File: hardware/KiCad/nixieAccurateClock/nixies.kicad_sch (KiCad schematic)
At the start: 7 parts, among them J17 Conn_02x05_Odd_Even

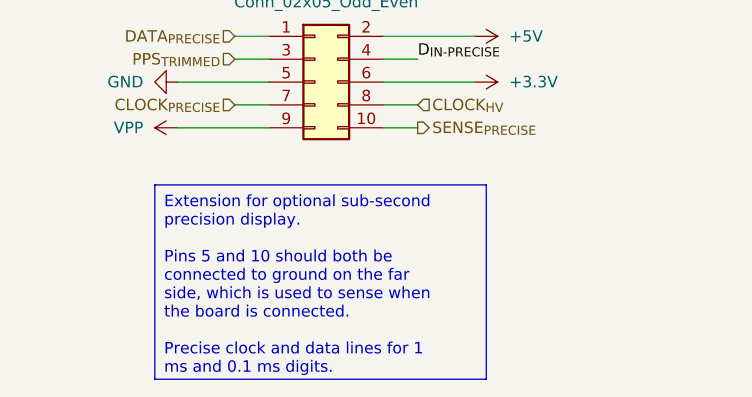
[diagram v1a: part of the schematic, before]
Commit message: Modify HV supply to attempt to solve weak IC
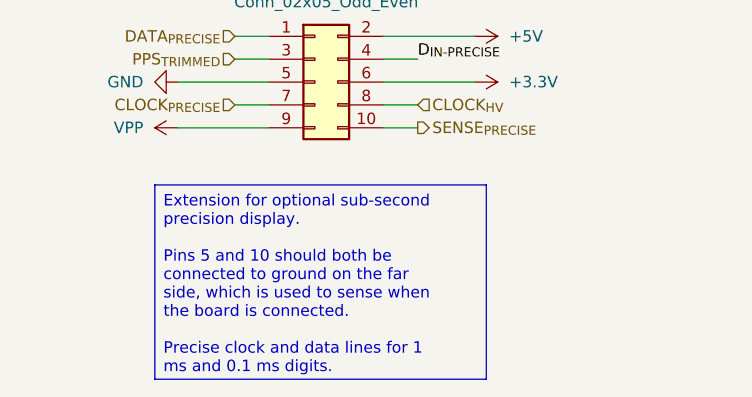
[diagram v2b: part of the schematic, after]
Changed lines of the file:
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@@
 (kicad_sch
-	(version 20231120)
+	(version 20250114)
 	(generator "eeschema")
-	(generator_version "8.0")
+	(generator_version "9.0")
 	(paper "A4")
 	(title_block
@@
 		(company "Paul Willis")
 	)
+	(text_box "Extension for optional sub-second precision display.\n\nPins 5 and 10 should both be connected to ground on the far side, which is used to sense when the board is connected.\n\nPrecise clock and data lines for 1 ms and 0.1 ms digits."
+		(exclude_from_sim no)
+		(at 27.94 147.32 0)
+		(size 36.83 21.59)
+		(margins 0.9525 0.9525 0.9525 0.9525)
+		(stroke
+			(width 0)
+			(type default)
+		)
+		(fill
+			(type none)
+		)
+		(effects
+			(font
+				(size 1.27 1.27)
+			)
+			(justify left top)
+		)
+	)
 	(junction
 		(at 162.56 93.98)
@@
 		)
 	)
-	(text_box "Extension for optional sub-second precision display.\n\nPins 5 and 10 should both be connected to ground on the far side, which is used to sense when the board is connected.\n\nPrecise clock and data lines for 1 ms and 0.1 ms digits."
-		(exclude_from_sim no)
-		(at 27.94 147.32 0)
-		(size 36.83 21.59)
-		(stroke
-			(width 0)
-			(type default)
-		)
-		(fill
-			(type none)
-		)
-		(effects
-			(font
-				(size 1.27 1.27)
-			)
-			(justify left top)
-		)
-	)
 	(label "DAISY_{HV-4}"
 		(at 67.31 104.14 0)
-		(fields_autoplaced yes)
 		(effects
 			(font
@@
 	(label "DAISY_{HV-1}"
 		(at 67.31 74.93 0)
-		(fields_autoplaced yes)
 		(effects
 			(font
@@
 	(label "DAISY_{HV-5}"
 		(at 132.08 104.14 0)
-		(fields_autoplaced yes)
 		(effects
 			(font
@@
 	(label "DAISY_{HV-3}"
 		(at 31.75 105.41 180)
-		(fields_autoplaced yes)
 		(effects
 			(font
@@
 	(label "D_{IN-PRECISE}"
 		(at 199.39 104.14 0)
-		(fields_autoplaced yes)
 		(effects
 			(font
@@
 	(label "DAISY_{HV-3}"
 		(at 196.85 74.93 0)
-		(fields_autoplaced yes)
 		(effects
 			(font
@@
 	(label "DAISY_{HV-2}"
 		(at 132.08 74.93 0)
-		(fields_autoplaced yes)
 		(effects
 			(font
@@
 	(label "D_{IN-PRECISE}"
 		(at 57.15 133.35 0)
-		(fields_autoplaced yes)
 		(effects
 			(font
@@
 		(shape input)
 		(at 161.29 69.85 180)
-		(fields_autoplaced yes)
 		(effects
 			(font
@@
 		(shape input)
 		(at 36.83 130.81 180)
-		(fields_autoplaced yes)
 		(effects
 			(font
@@
 		(shape output)
 		(at 57.15 140.97 0)
-		(fields_autoplaced yes)
 		(effects
 			(font
@@
 		(shape input)
 		(at 31.75 101.6 180)
-		(fields_autoplaced yes)
 		(effects
 			(font
@@
 		(shape input)
 		(at 96.52 99.06 180)
-		(fields_autoplaced yes)
 		(effects
 			(font
@@
 		(shape input)
 		(at 161.29 101.6 180)
-		(fields_autoplaced yes)
 		(effects
 			(font
@@
 		(shape input)
 		(at 31.75 72.39 180)
-		(fields_autoplaced yes)
 		(effects
 			(font
@@
 		(shape input)
 		(at 31.75 69.85 180)
-		(fields_autoplaced yes)
 		(effects
 			(font
@@
 		(shape output)
 		(at 199.39 106.68 0)
-		(fields_autoplaced yes)
 		(effects
 			(font
@@
 		(shape input)
 		(at 96.52 72.39 180)
-		(fields_autoplaced yes)
 		(effects
 			(font
@@
 		(shape input)
 		(at 57.15 138.43 0)
-		(fields_autoplaced yes)
 		(effects
 			(font
@@
 		(shape input)
 		(at 161.29 99.06 180)
-		(fields_autoplaced yes)
 		(effects
 			(font
@@
 		(shape input)
 		(at 31.75 99.06 180)
-		(fields_autoplaced yes)
 		(effects
 			(font
@@
 		(shape input)
 		(at 161.29 72.39 180)
-		(fields_autoplaced yes)
 		(effects
 			(font
@@
 		(shape input)
 		(at 31.75 74.93 180)
-		(fields_autoplaced yes)
 		(effects
 			(font
@@
 		(shape input)
 		(at 96.52 69.85 180)
-		(fields_autoplaced yes)
 		(effects
 			(font
@@
 		(shape input)
 		(at 36.83 138.43 180)
-		(fields_autoplaced yes)
 		(effects
 			(font
@@
 		(shape input)
 		(at 36.83 133.35 180)
-		(fields_autoplaced yes)
 		(effects
 			(font
@@
 		(shape input)
 		(at 96.52 101.6 180)
-		(fields_autoplaced yes)
-		(effects
-			(font
+		(effects
+			(font
